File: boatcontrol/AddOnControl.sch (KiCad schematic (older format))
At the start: 12 parts, among them J3901 Conn_01x01_Male, J3902 Conn_01x01_Male, J3903 Conn_02x20_Odd_Even Socket, U3901 MCP23017-E/SP

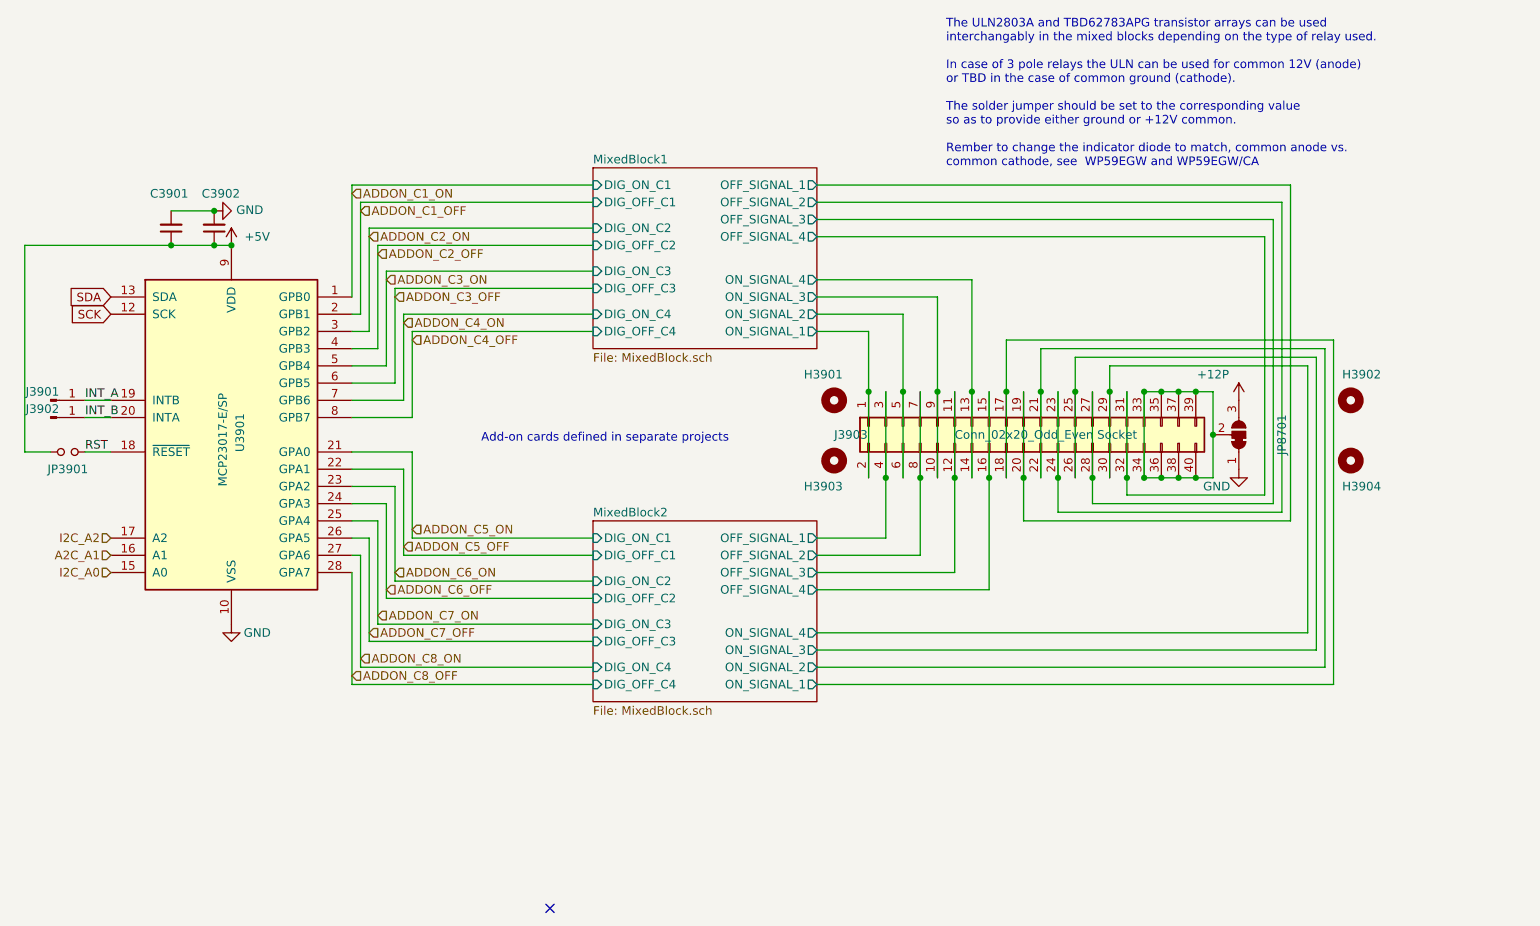
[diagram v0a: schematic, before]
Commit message: Deleting second heatsink
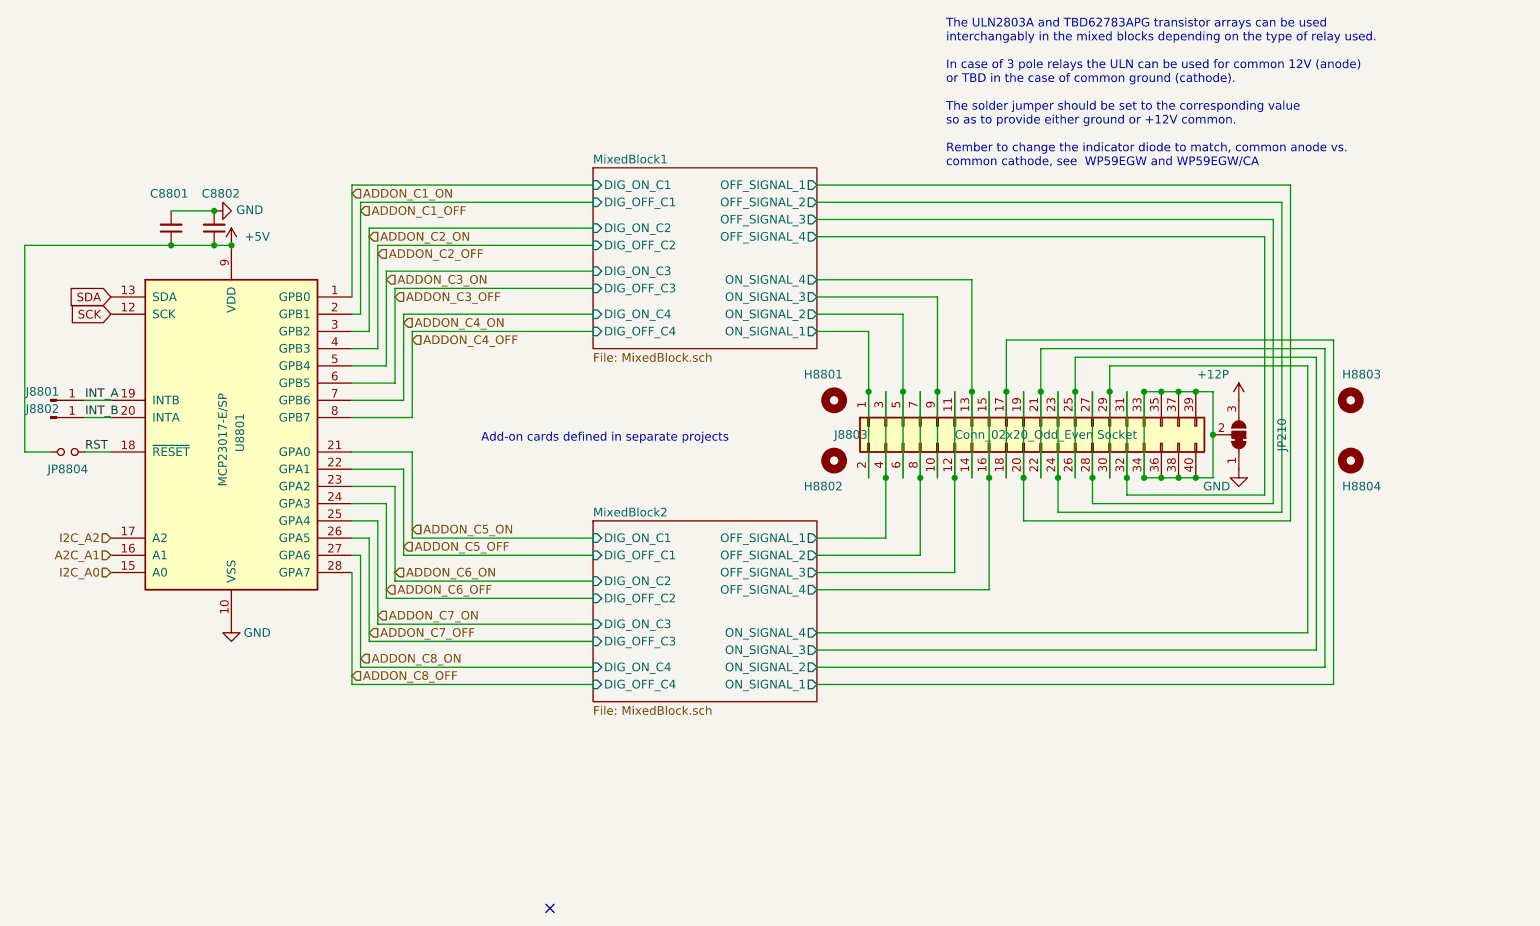
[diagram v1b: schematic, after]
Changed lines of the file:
@@
 $Descr A4 11693 8268
 encoding utf-8
-Sheet 87 97
+Sheet 76 97
 Title "Boat Control Hat"
 Date "2020-07-09"
@@
 AR Path="/626FCFE3/E142CC74" Ref="JP?"  Part="1"
 AR Path="/626FD005/E142CC74" Ref="JP?"  Part="1"
-F 0 "JP3901" H 3000 4050 50  0000 C CNN
+F 0 "JP8804" H 3000 4050 50  0000 C CNN
 F 1 "Jumper_NO_Small" H 3050 3850 50  0001 C CNN
 F 2 "Connector_PinHeader_2.54mm:PinHeader_1x02_P2.54mm_Vertical" H 3000 3950 50  0001 C CNN
@@
 AR Path="/626FCFE3/E142CCB8" Ref="#PWR?"  Part="1"
 AR Path="/626FD005/E142CCB8" Ref="#PWR?"  Part="1"
-F 0 "#PWR03903" H 3950 4700 50  0001 C CNN
+F 0 "#PWR0207" H 3950 4700 50  0001 C CNN
 F 1 "GND" H 4100 4900 50  0000 C CNN
 F 2 "" H 3950 4950 50  0001 C CNN
@@
 AR Path="/626FCFE3/E142CCC5" Ref="#PWR?"  Part="1"
 AR Path="/626FD005/E142CCC5" Ref="#PWR?"  Part="1"
-F 0 "#PWR03901" H 3950 2600 50  0001 C CNN
+F 0 "#PWR0208" H 3950 2600 50  0001 C CNN
 F 1 "+5V" H 4100 2800 50  0000 C CNN
 F 2 "" H 3950 2750 50  0001 C CNN
@@
 AR Path="/626FCFE3/E15696A6" Ref="H?"  Part="1"
 AR Path="/626FD005/E15696A6" Ref="H?"  Part="1"
-F 0 "H3902" H 10400 3800 50  0000 L CNN
+F 0 "H8803" H 10400 3800 50  0000 L CNN
 F 1 "MountingHole" V 10450 3750 50  0001 L CNN
 F 2 "MountingHole:MountingHole_3mm" H 10450 3650 50  0001 C CNN
@@
 AR Path="/626FCFE3/E156969A" Ref="J?"  Part="1"
 AR Path="/626FD005/E156969A" Ref="J?"  Part="1"
-F 0 "J3903" V 8600 4900 50  0000 R CNN
+F 0 "J8803" V 8600 4900 50  0000 R CNN
 F 1 "Conn_02x20_Odd_Even Socket" V 8600 4200 50  0000 R CNN
 F 2 "Connector_PinHeader_2.54mm:PinHeader_2x20_P2.54mm_Vertical" H 8550 3800 50  0001 C CNN
@@
 AR Path="/626FCFE3/E15696AC" Ref="H?"  Part="1"
 AR Path="/626FD005/E15696AC" Ref="H?"  Part="1"
-F 0 "H3901" V 7600 3600 50  0000 L CNN
+F 0 "H8801" V 7600 3600 50  0000 L CNN
 F 1 "MountingHole" H 7550 3605 50  0001 L CNN
 F 2 "MountingHole:MountingHole_3mm" H 7450 3650 50  0001 C CNN
@@
 AR Path="/626FCFE3/E15696A0" Ref="H?"  Part="1"
 AR Path="/626FD005/E15696A0" Ref="H?"  Part="1"
-F 0 "H3904" H 10400 3850 50  0000 L CNN
+F 0 "H8804" H 10400 3850 50  0000 L CNN
 F 1 "MountingHole" H 10550 3955 50  0001 L CNN
 F 2 "MountingHole:MountingHole_3mm" H 10450 4000 50  0001 C CNN
@@
 AR Path="/626FCFE3/61F82DD5" Ref="#PWR?"  Part="1"
 AR Path="/626FD005/61F82DD5" Ref="#PWR?"  Part="1"
-F 0 "#PWR0195" H 3850 2300 50  0001 C CNN
+F 0 "#PWR0210" H 3850 2300 50  0001 C CNN
 F 1 "GND" V 3855 2422 50  0000 R CNN
 F 2 "" H 3850 2550 50  0001 C CNN
@@
 AR Path="/626FCFE3/E15696B2" Ref="H?"  Part="1"
 AR Path="/626FD005/E15696B2" Ref="H?"  Part="1"
-F 0 "H3903" V 7300 3950 50  0000 L CNN
+F 0 "H8802" V 7300 3950 50  0000 L CNN
 F 1 "MountingHole" H 7550 3955 50  0001 L CNN
 F 2 "MountingHole:MountingHole_3mm" H 7450 4000 50  0001 C CNN
@@
 AR Path="/626FCFE3/E142CB7C" Ref="U?"  Part="1"
 AR Path="/626FD005/E142CB7C" Ref="U?"  Part="1"
-F 0 "U3901" V 4000 3750 50  0000 L CNN
+F 0 "U8801" V 4000 3750 50  0000 L CNN
 F 1 "MCP23017-E/SP" V 3900 3550 50  0000 L CNN
 F 2 "Package_DIP:DIP-28_W7.62mm" H 4150 2850 50  0001 L CNN
@@
 AR Path="/626FCFE3/E142CC93" Ref="J?"  Part="1"
 AR Path="/626FD005/E142CC93" Ref="J?"  Part="1"
-F 0 "J3901" H 2950 3700 50  0000 R CNN
+F 0 "J8801" H 2950 3700 50  0000 R CNN
 F 1 "Conn_01x01_Male" H 2872 3673 50  0001 R CNN
 F 2 "Connector_PinHeader_2.54mm:PinHeader_1x01_P2.54mm_Vertical" H 2900 3650 50  0001 C CNN
@@
 AR Path="/626FCFE3/E142CC7A" Ref="J?"  Part="1"
 AR Path="/626FD005/E142CC7A" Ref="J?"  Part="1"
-F 0 "J3902" H 2950 3800 50  0000 R CNN
+F 0 "J8802" H 2950 3800 50  0000 R CNN
 F 1 "Conn_01x01_Male" H 2872 3773 50  0001 R CNN
 F 2 "Connector_PinHeader_2.54mm:PinHeader_1x01_P2.54mm_Vertical" H 2900 3750 50  0001 C CNN
@@
 AR Path="/626FCFE3/60043DF4" Ref="C?"  Part="1"
 AR Path="/626FD005/60043DF4" Ref="C?"  Part="1"
-F 0 "C3901" H 3500 2450 50  0000 L CNN
+F 0 "C8801" H 3500 2450 50  0000 L CNN
 F 1 "10uF" H 3691 2605 50  0001 L CNN
 F 2 "Capacitor_THT:C_Disc_D7.5mm_W5.0mm_P5.00mm" H 3600 2650 50  0001 C CNN
@@
 AR Path="/626FCFE3/60043DFC" Ref="C?"  Part="1"
 AR Path="/626FD005/60043DFC" Ref="C?"  Part="1"
-F 0 "C3902" H 3700 2450 50  0000 L CNN
+F 0 "C8802" H 3700 2450 50  0000 L CNN
 F 1 "0.1uF" H 3941 2605 50  0001 L CNN
 F 2 "Capacitor_THT:C_Disc_D7.5mm_W5.0mm_P5.00mm" H 3850 2650 50  0001 C CNN
@@
 AR Path="/626FCFE3/60593EAA" Ref="JP?"  Part="1"
 AR Path="/626FD005/60593EAA" Ref="JP?"  Part="1"
-F 0 "JP8701" H 9800 4100 50  0000 C CNN
+F 0 "JP210" H 9800 4100 50  0000 C CNN
 F 1 "SolderJumper_3_Bridged12" H 9800 3964 50  0001 C CNN
 F 2 "BoatControl:SolderJumper-3_P1.3mm_Open_RoundedPad3.0x4.5mm_NumberLabels" H 9800 3850 50  0001 C CNN
@@
 AR Path="/626FCFE3/E16C27B4" Ref="#PWR?"  Part="1"
 AR Path="/626FD005/E16C27B4" Ref="#PWR?"  Part="1"
-F 0 "#PWR03902" H 9800 3800 50  0001 C CNN
+F 0 "#PWR0209" H 9800 3800 50  0001 C CNN
 F 1 "GND" H 9750 3950 50  0000 R CNN
 F 2 "" H 9800 4050 50  0001 C CNN
@@
 AR Path="/626FCFE3/605ACD99" Ref="#PWR?"  Part="1"
 AR Path="/626FD005/605ACD99" Ref="#PWR?"  Part="1"
-F 0 "#PWR0238" H 9800 3500 50  0001 C CNN
+F 0 "#PWR0237" H 9800 3500 50  0001 C CNN
 F 1 "+12P" H 9650 3800 50  0000 C CNN
 F 2 "" H 9800 3650 50  0001 C CNN

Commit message: Sorted Caps
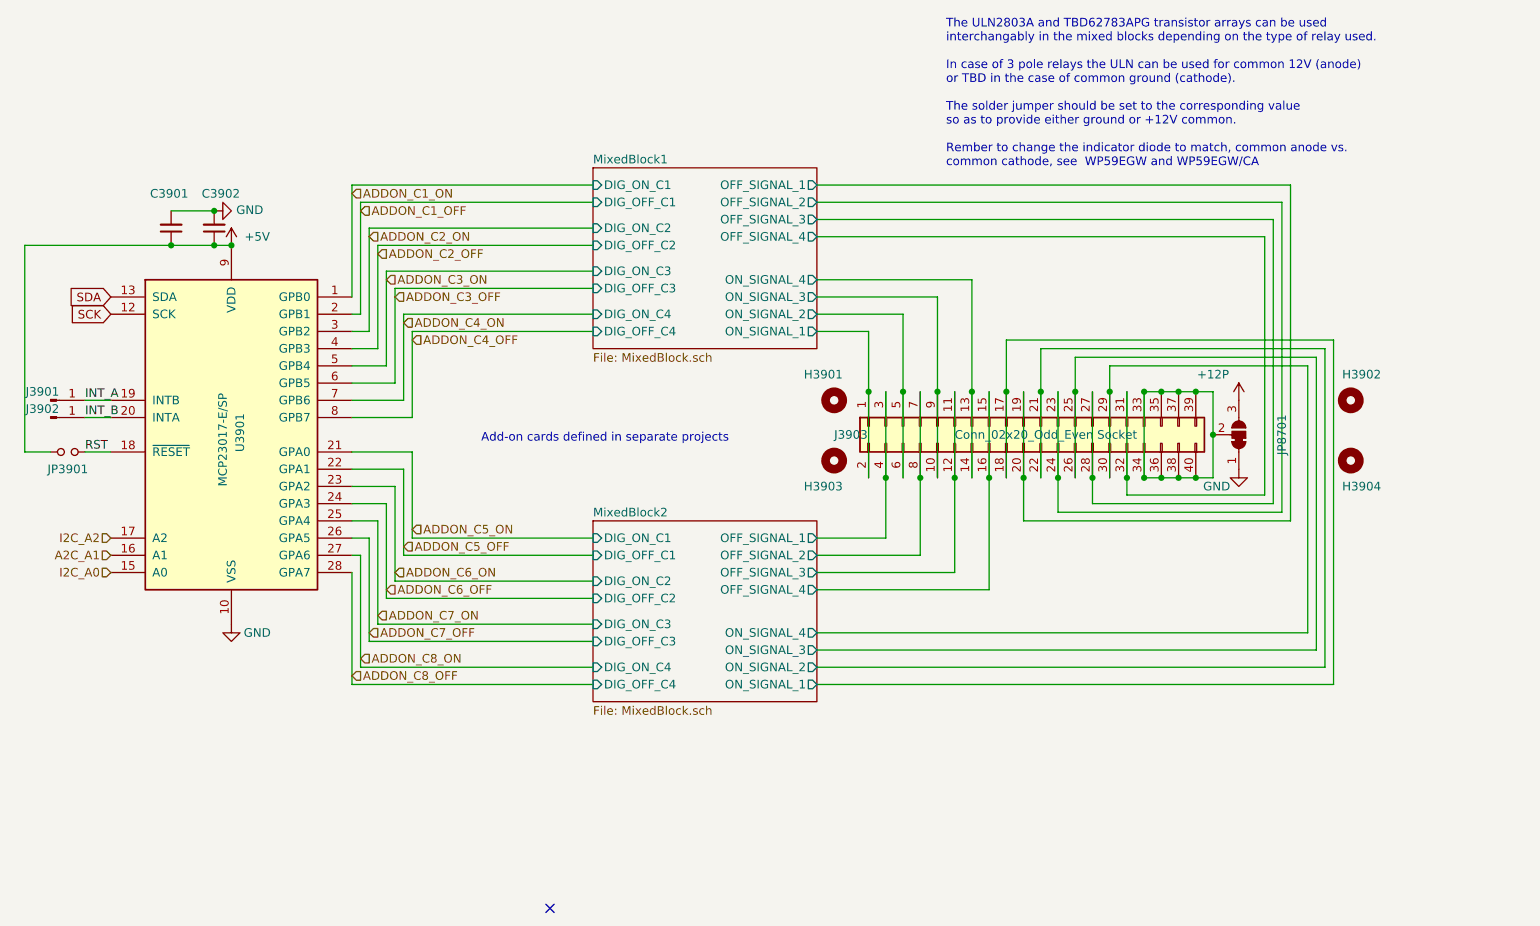
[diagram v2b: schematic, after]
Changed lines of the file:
@@
 AR Path="/626FCFE3/E142CC74" Ref="JP?"  Part="1"
 AR Path="/626FD005/E142CC74" Ref="JP?"  Part="1"
-F 0 "JP8804" H 3000 4050 50  0000 C CNN
+F 0 "JP3901" H 3000 4050 50  0000 C CNN
 F 1 "Jumper_NO_Small" H 3050 3850 50  0001 C CNN
 F 2 "Connector_PinHeader_2.54mm:PinHeader_1x02_P2.54mm_Vertical" H 3000 3950 50  0001 C CNN
@@
 AR Path="/626FCFE3/E142CCB8" Ref="#PWR?"  Part="1"
 AR Path="/626FD005/E142CCB8" Ref="#PWR?"  Part="1"
-F 0 "#PWR0207" H 3950 4700 50  0001 C CNN
+F 0 "#PWR03903" H 3950 4700 50  0001 C CNN
 F 1 "GND" H 4100 4900 50  0000 C CNN
 F 2 "" H 3950 4950 50  0001 C CNN
@@
 AR Path="/626FCFE3/E142CCC5" Ref="#PWR?"  Part="1"
 AR Path="/626FD005/E142CCC5" Ref="#PWR?"  Part="1"
-F 0 "#PWR0208" H 3950 2600 50  0001 C CNN
+F 0 "#PWR03901" H 3950 2600 50  0001 C CNN
 F 1 "+5V" H 4100 2800 50  0000 C CNN
 F 2 "" H 3950 2750 50  0001 C CNN
@@
 AR Path="/626FCFE3/E15696A6" Ref="H?"  Part="1"
 AR Path="/626FD005/E15696A6" Ref="H?"  Part="1"
-F 0 "H8803" H 10400 3800 50  0000 L CNN
+F 0 "H3902" H 10400 3800 50  0000 L CNN
 F 1 "MountingHole" V 10450 3750 50  0001 L CNN
 F 2 "MountingHole:MountingHole_3mm" H 10450 3650 50  0001 C CNN
@@
 AR Path="/626FCFE3/E156969A" Ref="J?"  Part="1"
 AR Path="/626FD005/E156969A" Ref="J?"  Part="1"
-F 0 "J8803" V 8600 4900 50  0000 R CNN
+F 0 "J3903" V 8600 4900 50  0000 R CNN
 F 1 "Conn_02x20_Odd_Even Socket" V 8600 4200 50  0000 R CNN
 F 2 "Connector_PinHeader_2.54mm:PinHeader_2x20_P2.54mm_Vertical" H 8550 3800 50  0001 C CNN
@@
 AR Path="/626FCFE3/E15696AC" Ref="H?"  Part="1"
 AR Path="/626FD005/E15696AC" Ref="H?"  Part="1"
-F 0 "H8801" V 7600 3600 50  0000 L CNN
+F 0 "H3901" V 7600 3600 50  0000 L CNN
 F 1 "MountingHole" H 7550 3605 50  0001 L CNN
 F 2 "MountingHole:MountingHole_3mm" H 7450 3650 50  0001 C CNN
@@
 AR Path="/626FCFE3/E15696A0" Ref="H?"  Part="1"
 AR Path="/626FD005/E15696A0" Ref="H?"  Part="1"
-F 0 "H8804" H 10400 3850 50  0000 L CNN
+F 0 "H3904" H 10400 3850 50  0000 L CNN
 F 1 "MountingHole" H 10550 3955 50  0001 L CNN
 F 2 "MountingHole:MountingHole_3mm" H 10450 4000 50  0001 C CNN
@@
 AR Path="/626FCFE3/61F82DD5" Ref="#PWR?"  Part="1"
 AR Path="/626FD005/61F82DD5" Ref="#PWR?"  Part="1"
-F 0 "#PWR0210" H 3850 2300 50  0001 C CNN
+F 0 "#PWR0195" H 3850 2300 50  0001 C CNN
 F 1 "GND" V 3855 2422 50  0000 R CNN
 F 2 "" H 3850 2550 50  0001 C CNN
@@
 AR Path="/626FCFE3/E15696B2" Ref="H?"  Part="1"
 AR Path="/626FD005/E15696B2" Ref="H?"  Part="1"
-F 0 "H8802" V 7300 3950 50  0000 L CNN
+F 0 "H3903" V 7300 3950 50  0000 L CNN
 F 1 "MountingHole" H 7550 3955 50  0001 L CNN
 F 2 "MountingHole:MountingHole_3mm" H 7450 4000 50  0001 C CNN
@@
 AR Path="/626FCFE3/E142CB7C" Ref="U?"  Part="1"
 AR Path="/626FD005/E142CB7C" Ref="U?"  Part="1"
-F 0 "U8801" V 4000 3750 50  0000 L CNN
+F 0 "U3901" V 4000 3750 50  0000 L CNN
 F 1 "MCP23017-E/SP" V 3900 3550 50  0000 L CNN
 F 2 "Package_DIP:DIP-28_W7.62mm" H 4150 2850 50  0001 L CNN
@@
 AR Path="/626FCFE3/E142CC93" Ref="J?"  Part="1"
 AR Path="/626FD005/E142CC93" Ref="J?"  Part="1"
-F 0 "J8801" H 2950 3700 50  0000 R CNN
+F 0 "J3901" H 2950 3700 50  0000 R CNN
 F 1 "Conn_01x01_Male" H 2872 3673 50  0001 R CNN
 F 2 "Connector_PinHeader_2.54mm:PinHeader_1x01_P2.54mm_Vertical" H 2900 3650 50  0001 C CNN
@@
 AR Path="/626FCFE3/E142CC7A" Ref="J?"  Part="1"
 AR Path="/626FD005/E142CC7A" Ref="J?"  Part="1"
-F 0 "J8802" H 2950 3800 50  0000 R CNN
+F 0 "J3902" H 2950 3800 50  0000 R CNN
 F 1 "Conn_01x01_Male" H 2872 3773 50  0001 R CNN
 F 2 "Connector_PinHeader_2.54mm:PinHeader_1x01_P2.54mm_Vertical" H 2900 3750 50  0001 C CNN
@@
 AR Path="/626FCFE3/60043DF4" Ref="C?"  Part="1"
 AR Path="/626FD005/60043DF4" Ref="C?"  Part="1"
-F 0 "C8801" H 3500 2450 50  0000 L CNN
+F 0 "C3901" H 3500 2450 50  0000 L CNN
 F 1 "10uF" H 3691 2605 50  0001 L CNN
 F 2 "Capacitor_THT:C_Disc_D7.5mm_W5.0mm_P5.00mm" H 3600 2650 50  0001 C CNN
@@
 AR Path="/626FCFE3/60043DFC" Ref="C?"  Part="1"
 AR Path="/626FD005/60043DFC" Ref="C?"  Part="1"
-F 0 "C8802" H 3700 2450 50  0000 L CNN
+F 0 "C3902" H 3700 2450 50  0000 L CNN
 F 1 "0.1uF" H 3941 2605 50  0001 L CNN
 F 2 "Capacitor_THT:C_Disc_D7.5mm_W5.0mm_P5.00mm" H 3850 2650 50  0001 C CNN
@@
 AR Path="/626FCFE3/60593EAA" Ref="JP?"  Part="1"
 AR Path="/626FD005/60593EAA" Ref="JP?"  Part="1"
-F 0 "JP210" H 9800 4100 50  0000 C CNN
+F 0 "JP8701" H 9800 4100 50  0000 C CNN
 F 1 "SolderJumper_3_Bridged12" H 9800 3964 50  0001 C CNN
 F 2 "BoatControl:SolderJumper-3_P1.3mm_Open_RoundedPad3.0x4.5mm_NumberLabels" H 9800 3850 50  0001 C CNN
@@
 AR Path="/626FCFE3/E16C27B4" Ref="#PWR?"  Part="1"
 AR Path="/626FD005/E16C27B4" Ref="#PWR?"  Part="1"
-F 0 "#PWR0209" H 9800 3800 50  0001 C CNN
+F 0 "#PWR03902" H 9800 3800 50  0001 C CNN
 F 1 "GND" H 9750 3950 50  0000 R CNN
 F 2 "" H 9800 4050 50  0001 C CNN
@@
 AR Path="/626FCFE3/605ACD99" Ref="#PWR?"  Part="1"
 AR Path="/626FD005/605ACD99" Ref="#PWR?"  Part="1"
-F 0 "#PWR0237" H 9800 3500 50  0001 C CNN
+F 0 "#PWR0238" H 9800 3500 50  0001 C CNN
 F 1 "+12P" H 9650 3800 50  0000 C CNN
 F 2 "" H 9800 3650 50  0001 C CNN
